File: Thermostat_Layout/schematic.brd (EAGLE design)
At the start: 100 x 69.8 mm, 31 parts, among them IC1 LM50, IC2 MCP23017SO, IC3 MCP23017SO, Q1 10 MHz, U1 ATMEGA328P-AU, U2 DS3231M+, U3 AT25DF021-SSH-B, U4 VO14642AT, U5 VO14642AT, U6 VO14642AT

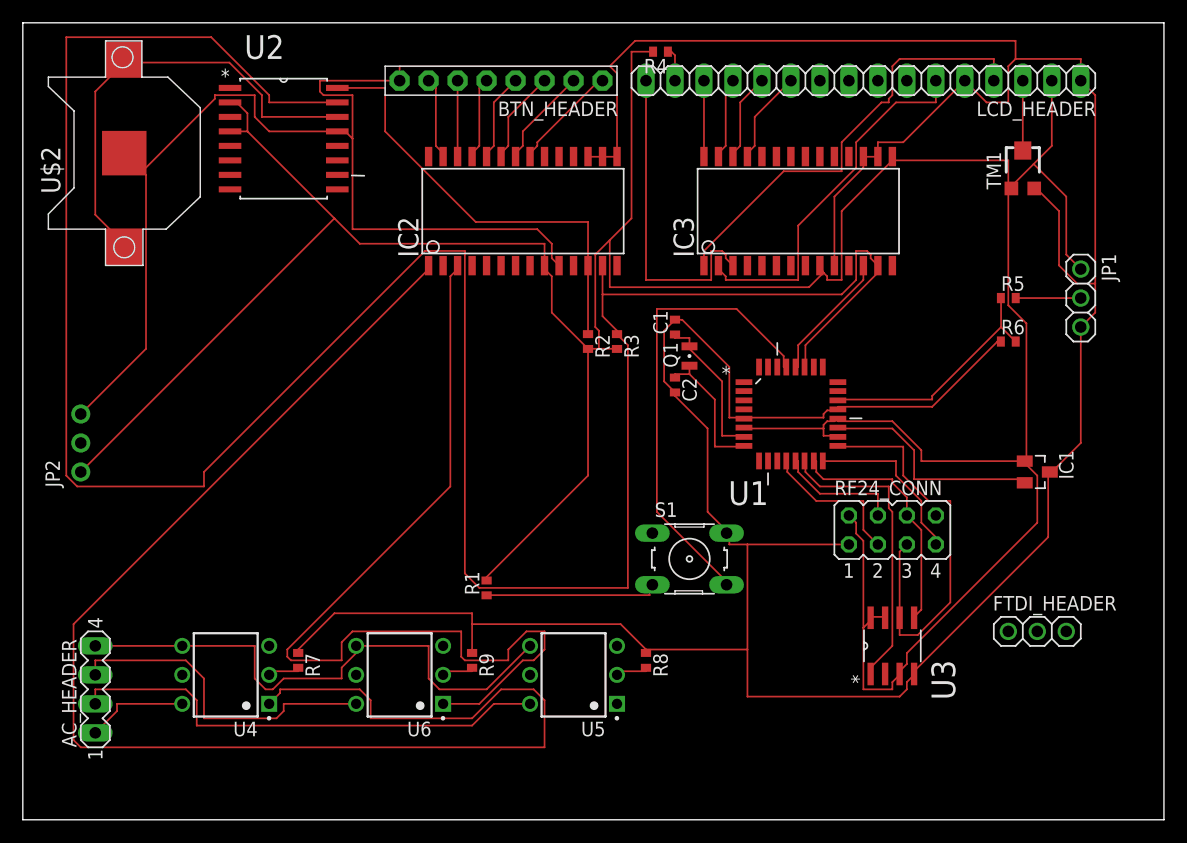
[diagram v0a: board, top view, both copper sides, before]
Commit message: Clean up schematic and board
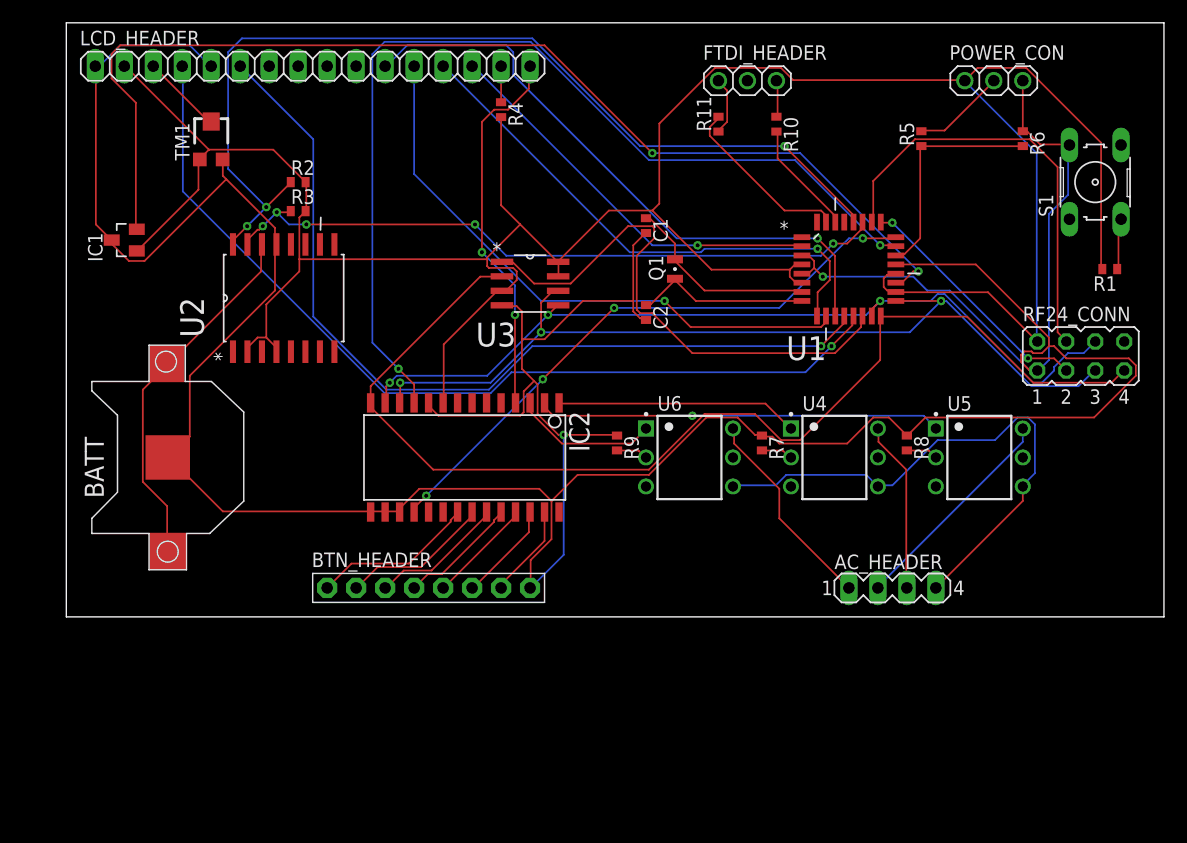
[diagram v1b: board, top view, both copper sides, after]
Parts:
- removed IC3: MCP23017SO, microchip:SO28W
- removed JP1: (no value), adafruit:1X03
- removed JP2: (no value), adafruit:1X03-CLEANBIG
- removed U$2: cr1220, adafruit:CR1220-SMD
- added BATT: cr1220, adafruit:CR1220-SMD
- added POWER_CON: (no value), adafruit:1X03
- added R10, R11: 1k, resistor:R0402
- IC2: value MCP23017SO -> MCP23S17SO
- moved IC1 82.5 mm to (8.89, 61.0), turned to 90 degrees
- moved TM1 71.2 mm to (16.5, 69.8)
- moved AC_HEADER 70.4 mm to (76.2, 30.5), turned to 0 degrees
- moved R1 61.3 mm to (95.2, 58.4), turned to 180 degrees
- moved U4 56.6 mm to (71.1, 41.9), turned to 0 degrees
- moved FTDI_HEADER 54.5 mm to (63.5, 74.9)
- moved S1 48.5 mm to (94.0, 66.0), turned to 90 degrees
- moved LCD_HEADER 48.3 mm to (25.4, 76.2), turned to 0 degrees
- moved BTN_HEADER 44.9 mm to (35.6, 30.5), turned to 0 degrees
- moved U3 44.9 mm to (44.5, 57.1), turned to 0 degrees
- moved R7 44.9 mm to (64.8, 43.2)
- moved U5 40.3 mm to (83.8, 41.9), turned to 0 degrees
- moved U6 31.8 mm to (58.4, 41.9), turned to 0 degrees
- moved R3 30.2 mm to (24.1, 63.5), turned to 0 degrees
- moved R8 29.8 mm to (77.5, 43.2)
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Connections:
- net DWN_TEMP_BTN renamed DWN_BTN
- net UP_TEMP_BTN renamed UP_BTN
- removed net EXP_INTA: IC2.20, U1.32
- removed net VCC_2: U1.4
- new net EXP_INT: IC2.20
- new net N$10: R11.2, U1.31
- new net N$13: U1.1
- new net N$9: R10.2, U1.30
- net +3V3: now also POWER_CON.1, U1.4; no longer IC3.15, IC3.9, JP1.1, JP2.1
- net +9V: now also POWER_CON.2; no longer JP1.2
- net EXP_CS: now also IC2.11, U1.23; no longer U1.11
- net EXP_RST: now also U1.24; no longer U1.10
- net FAN_HOT: now also AC_HEADER.1; no longer AC_HEADER.3
- net GND: now also BATT.-, POWER_CON.3, U1.3; no longer IC3.10, IC3.16, IC3.17, JP1.3, JP2.3, U$2.-
- net HEAT_HOT: now also AC_HEADER.3; no longer AC_HEADER.1
- net LCD_D0: now also LCD_HEADER.7; no longer IC3.21
- net LCD_D1: now also LCD_HEADER.8; no longer IC3.22
- net LCD_D2: now also LCD_HEADER.9; no longer IC3.23
- net LCD_D3: now also LCD_HEADER.10; no longer IC3.24
- net LCD_D4: now also U1.11; no longer IC3.25
- net LCD_D5: now also U1.10; no longer IC3.26
- net LCD_D6: now also U1.9; no longer IC3.27
- net LCD_D7: now also U1.2; no longer IC3.28
- net LCD_EN: now also U1.12; no longer IC3.2
- net LCD_LED: now also IC2.4; no longer IC3.3
- net LCD_RS: now also U1.13; no longer IC3.1
- net MISO: now also IC2.14
- net MOSI: now also IC2.13
- net N$8: now also BATT.+$1, BATT.+$2; no longer U$2.+$1, U$2.+$2
- net RF_CE: now also U1.25; no longer U1.12
- net RF_CS: now also U1.26; no longer U1.13
- net SCK: now also IC2.12
- net SCL: no longer IC2.12, IC3.12
- net SDA: no longer IC2.13, IC3.13
- net UC_RST: no longer U1.29
- net UC_RX: now also R10.1; no longer U1.30
- net UC_TX: now also R11.1; no longer U1.31
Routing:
- net SDA: track 221.3 -> 59.8 mm, vias 0 -> 5
- net HEAT_ON: track 128.4 -> 21.2 mm
- net EXP_CS: track 0.00 -> 85.9 mm, vias 0 -> 2
- net GND: track 417.3 -> 332.5 mm, vias 0 -> 2
- net MISO: track 15.2 -> 98.2 mm
- net ANA_TEMP: track 20.0 -> 97.9 mm, vias 0 -> 2
- net FAN_ON: track 81.5 -> 12.7 mm
- net +3V3: track 308.1 -> 239.6 mm
- net MOSI: track 21.6 -> 74.7 mm, vias 0 -> 3
- net EXP_RST: track 0.00 -> 52.5 mm, vias 0 -> 4
- net LCD_D4: track 8.23 -> 54.3 mm, vias 0 -> 1
- net LCD_EN: track 32.4 -> 76.8 mm, vias 0 -> 1
- net LCD_D5: track 7.70 -> 51.8 mm, vias 0 -> 1
- net SCK: track 36.1 -> 77.8 mm, vias 0 -> 3
- net LCD_RS: track 38.7 -> 80.4 mm, vias 0 -> 1
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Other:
- board size 100 x 69.8 mm -> 96.2 x 52.1 mm
